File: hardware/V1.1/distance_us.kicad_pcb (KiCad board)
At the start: 2 copper layers, 20 x 45 mm, 29 parts, among them P1 CON-SENSOR, P2 CONN_4, Q1 2N7002P, Q2 2N7002P, U1 M24C64, U2 LMV358LI, U3 DRILL, U4 DRILL, U5 DRILL, U6 DRILL

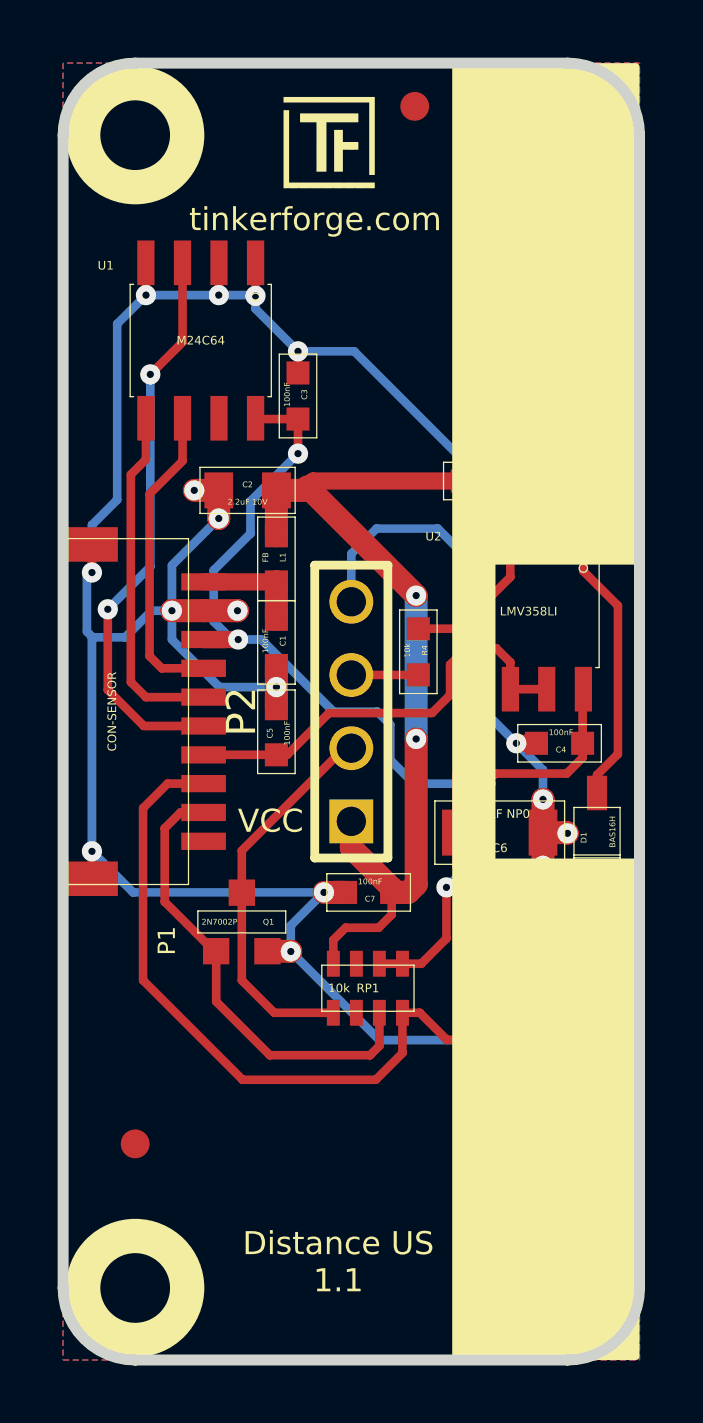
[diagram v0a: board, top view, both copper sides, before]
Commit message: Add 3d information (final)
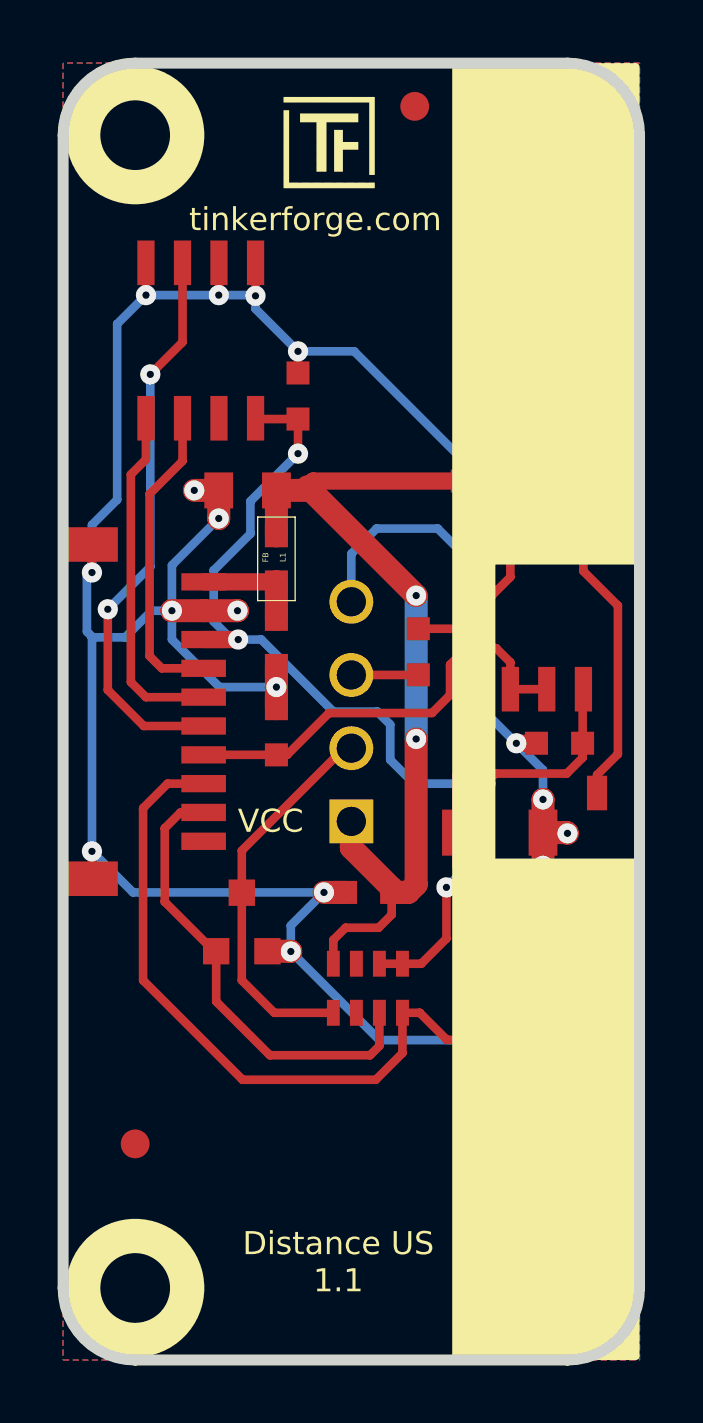
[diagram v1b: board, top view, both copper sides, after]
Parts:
- added P2: CONN_4, kicad-libraries:distanceUS_overlay, F.Cu at (52.9, 42.3)
- C1, C3, C4, C5, C7: footprint kicad-libraries:0603 -> kicad-libraries:C0603
- C2: footprint kicad-libraries:0805 -> kicad-libraries:C0805
- C6: footprint kicad-libraries:1206 -> kicad-libraries:C1206
- R1, R2, R3, R4: footprint kicad-libraries:0603 -> kicad-libraries:R0603
- VAL: footprint kicad-libraries:WEEE_7mm_back -> kicad-libraries:WEEE_7mm
- turned VAL to 180 degrees
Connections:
- P1 pad 10: (no net) -> Net-(P1-Pad10)
- RP1 pad 2: (no net) -> Net-(RP1-Pad2)
- RP1 pad 7: (no net) -> Net-(RP1-Pad7)
- U1 pad 7: (no net) -> Net-(U1-Pad7)
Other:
- outline, holes or cut-outs redrawn
